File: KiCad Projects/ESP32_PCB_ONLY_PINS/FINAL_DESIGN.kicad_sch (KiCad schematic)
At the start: 62 parts, among them J1 Screw_Terminal_01x02, J2 TB010-508-P19BK, J3 Conn_01x19_Socket, J4 TB010-508-P19BK, J5 Conn_01x19_Socket, Q1 AO3401A, U1 LM2596S-5

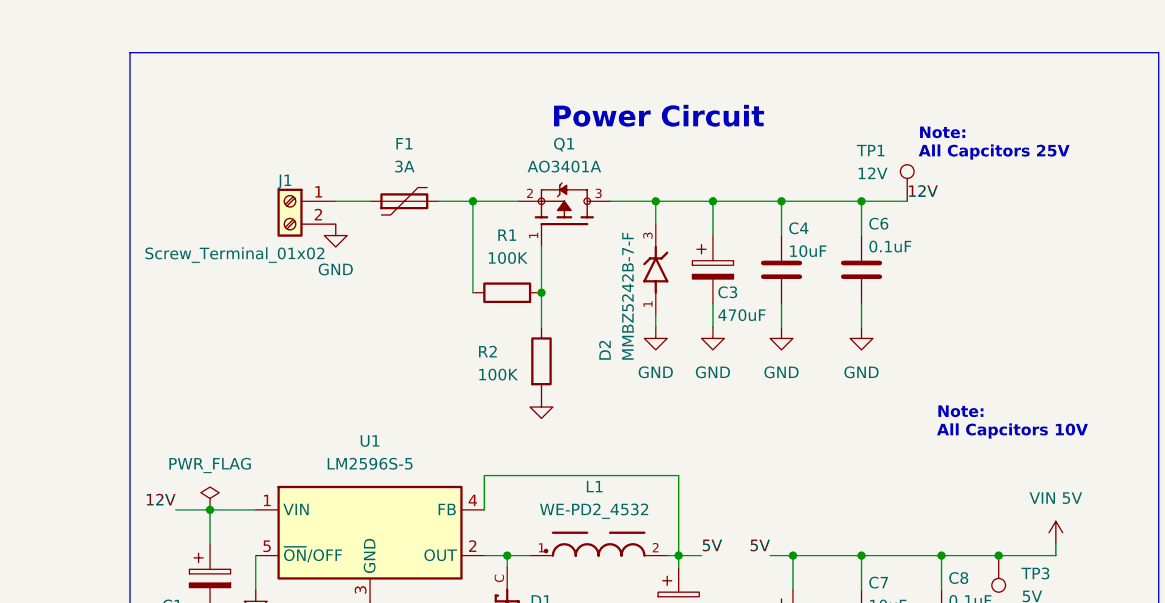
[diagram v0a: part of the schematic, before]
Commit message: work
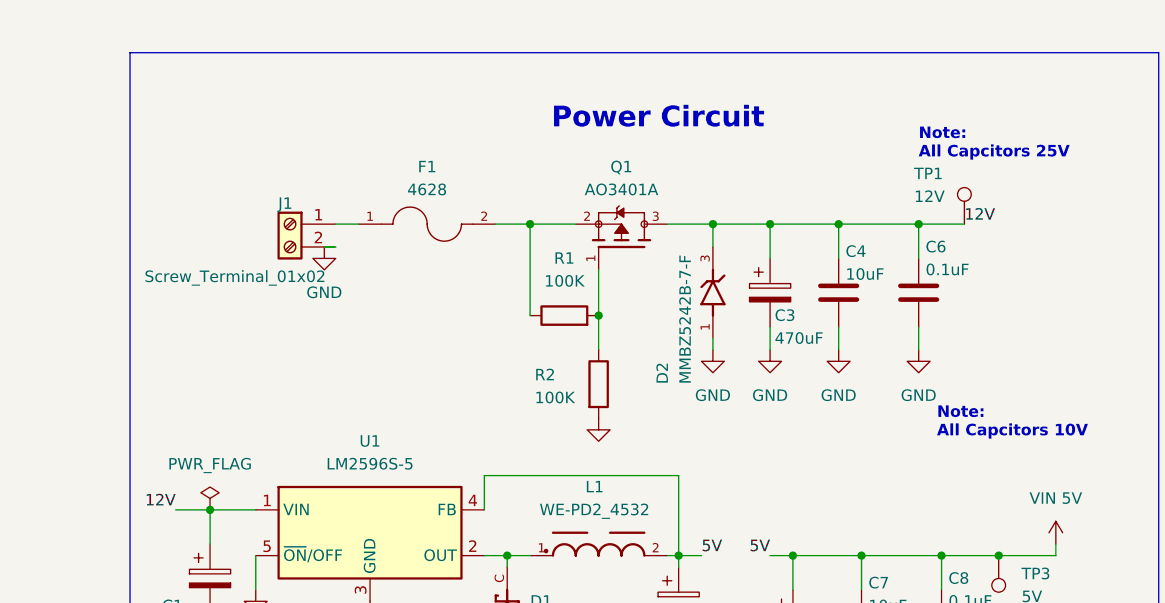
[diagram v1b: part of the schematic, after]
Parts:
- removed F1: 3A, Fuse:FuseHolder_Blade_ATO_Littelfuse_FLR_178.6165, symbol Device:Polyfuse
- added F1: 4628, CATRIDGE_FUSE:FUSE_4628, symbol 4628:4628
- C4, C6, C7, C8: footprint Capacitor_SMD:C_0805_2012Metric -> Capacitor_SMD:C_1206_3216Metric
- R1, R2: footprint Resistor_SMD:R_0805_2012Metric_Pad1.20x1.40mm_HandSolder -> Resistor_SMD:R_1206_3216Metric
- R10, R11, R12, R13, R14, R15, R16, R17, R18, R19, R20, R21, R3, R4, R5, R6, R7, R8, R9: footprint Resistor_SMD:R_0805_2012Metric -> Resistor_SMD:R_1206_3216Metric
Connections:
- net at Q1.2, R1.1: now also F1.2
- net at J1.1 (Pin_1): now also F1.1
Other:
- moved on the sheet: C3, C4, C6, D2, J1, Q1, R1, R2, TP1
